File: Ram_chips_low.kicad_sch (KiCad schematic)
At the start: 10 parts, among them U25 MM5280, U26 MM5280, U27 MM5280, U28 MM5280, U40 MM5280, U41 MM5280, U42 MM5280, U43 MM5280, U6 74LS04, U7 74LS173

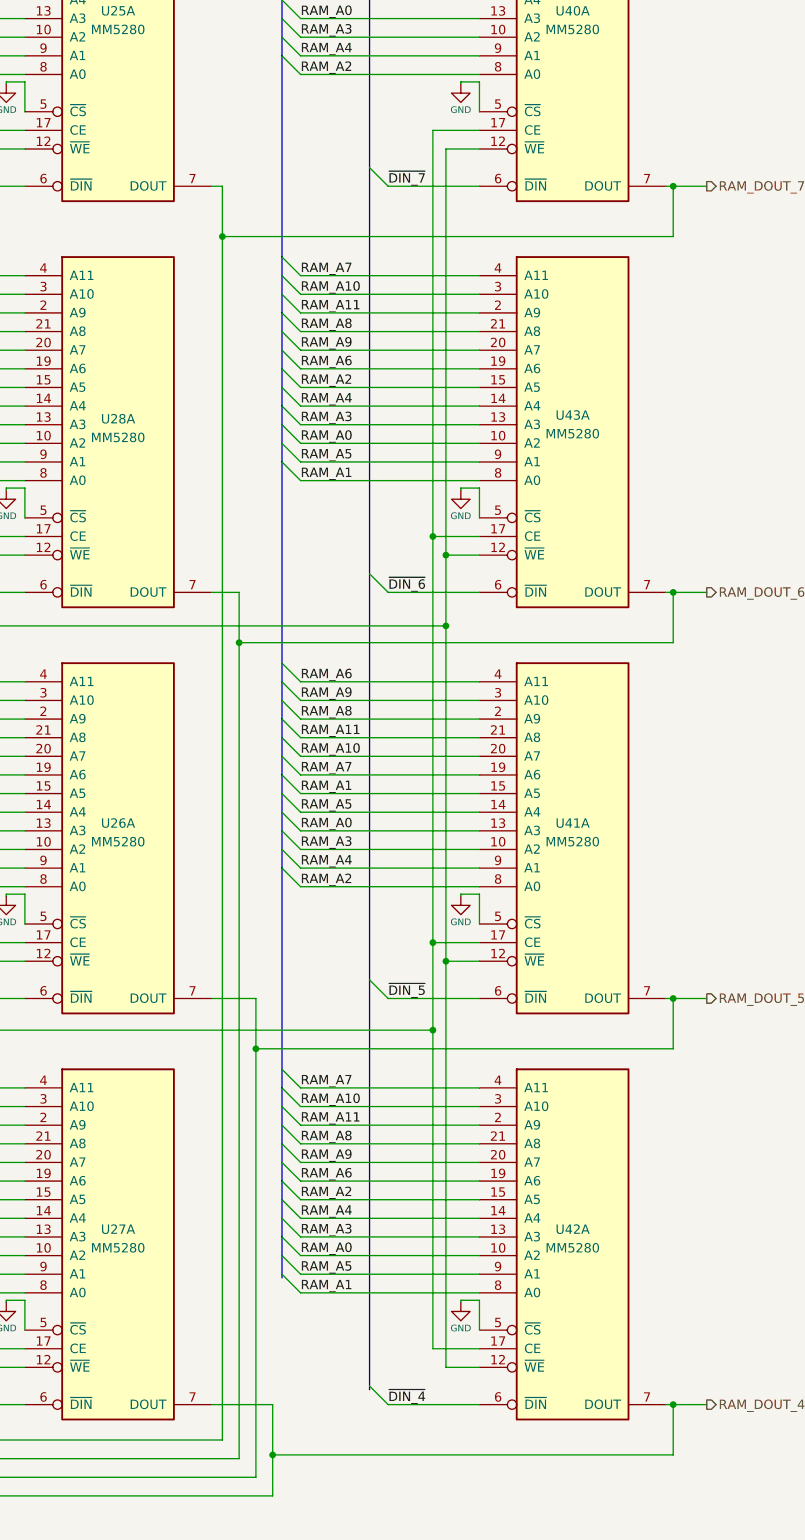
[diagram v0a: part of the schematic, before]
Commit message: Routing completed
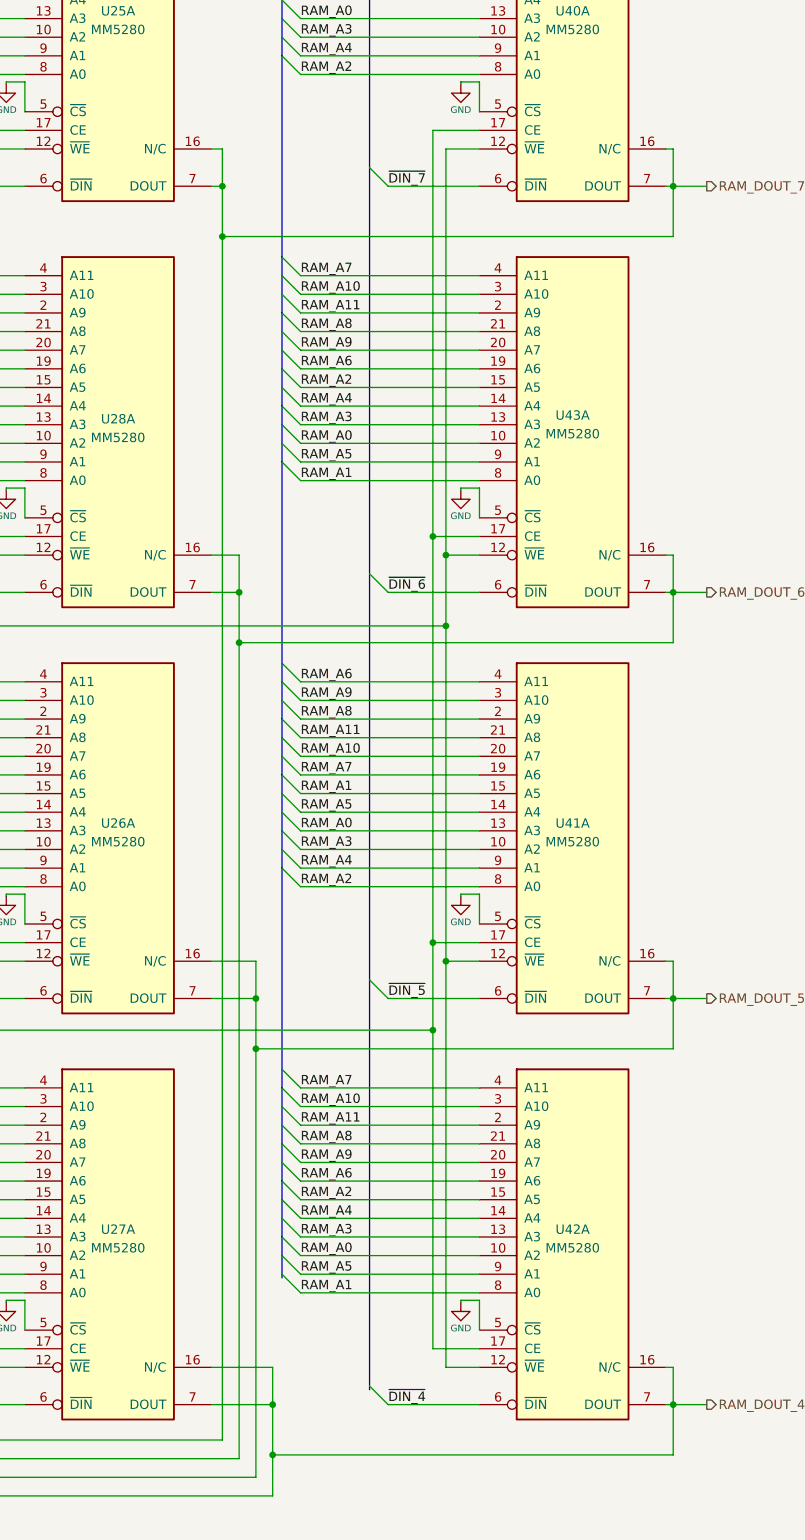
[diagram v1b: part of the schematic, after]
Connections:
- net RAM_DOUT_4: now also U27.16 (N/C), U42.16 (N/C)
- net RAM_DOUT_5: now also U26.16 (N/C), U41.16 (N/C)
- net RAM_DOUT_6: now also U28.16 (N/C), U43.16 (N/C)
- net RAM_DOUT_7: now also U25.16 (N/C), U40.16 (N/C)
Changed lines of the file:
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@@
   (junction (at 146.05 127.508) (diameter 0) (color 0 0 0 0)
   )
+  (junction (at 120.142 178.308) (diameter 0) (color 0 0 0 0)
+  )
+  (junction (at 117.856 122.936) (diameter 0) (color 0 0 0 0)
+  )
   (junction (at 120.142 185.166) (diameter 0) (color 0 0 0 0)
   )
+  (junction (at 122.428 233.68) (diameter 0) (color 0 0 0 0)
+  )
   (junction (at 81.534 115.316) (diameter 0) (color 0 0 0 0)
   )
@@
   (junction (at 33.274 195.072) (diameter 0) (color 0 0 0 0)
   )
+  (junction (at 115.57 67.564) (diameter 0) (color 0 0 0 0)
+  )
   (junction (at 83.312 117.856) (diameter 0) (color 0 0 0 0)
   )
@@
     (stroke (width 0) (type default))
   )
+  (wire (pts (xy 120.142 173.228) (xy 120.142 178.308))
+    (stroke (width 0) (type default))
+  )
   (wire (pts (xy 83.312 173.228) (xy 88.646 173.228))
     (stroke (width 0) (type default))
@@
     (stroke (width 0) (type default))
   )
+  (wire (pts (xy 177.038 173.228) (xy 177.038 178.308))
+    (stroke (width 0) (type default))
+  )
   (wire (pts (xy 126.238 82.296) (xy 150.622 82.296))
     (stroke (width 0) (type default))
   )
+  (wire (pts (xy 177.038 62.484) (xy 177.038 67.564))
+    (stroke (width 0) (type default))
+  )
   (bus (pts (xy 60.452 208.28) (xy 60.452 210.82))
     (stroke (width 0) (type default))
@@
     (stroke (width 0) (type default))
   )
+  (wire (pts (xy 176.022 173.228) (xy 177.038 173.228))
+    (stroke (width 0) (type default))
+  )
   (bus (pts (xy 60.452 77.216) (xy 60.452 79.756))
     (stroke (width 0) (type default))
@@
     (stroke (width 0) (type default))
   )
+  (wire (pts (xy 176.022 228.6) (xy 177.038 228.6))
+    (stroke (width 0) (type default))
+  )
   (bus (pts (xy 60.452 102.616) (xy 60.452 105.156))
     (stroke (width 0) (type default))
@@
     (stroke (width 0) (type default))
   )
+  (wire (pts (xy 114.046 228.6) (xy 122.428 228.6))
+    (stroke (width 0) (type default))
+  )
   (wire (pts (xy 62.992 195.58) (xy 88.646 195.58))
     (stroke (width 0) (type default))
@@
     (stroke (width 0) (type default))
   )
+  (wire (pts (xy 115.57 62.484) (xy 115.57 67.564))
+    (stroke (width 0) (type default))
+  )
   (bus (pts (xy 60.452 29.464) (xy 60.452 30.988))
     (stroke (width 0) (type default))
@@
     (stroke (width 0) (type default))
   )
+  (wire (pts (xy 176.022 62.484) (xy 177.038 62.484))
+    (stroke (width 0) (type default))
+  )
   (bus (pts (xy 123.698 203.2) (xy 123.698 205.74))
     (stroke (width 0) (type default))
@@
     (stroke (width 0) (type default))
   )
+  (wire (pts (xy 114.046 117.856) (xy 117.856 117.856))
+    (stroke (width 0) (type default))
+  )
   (wire (pts (xy 62.992 147.828) (xy 88.646 147.828))
     (stroke (width 0) (type default))
@@
     (stroke (width 0) (type default))
   )
+  (wire (pts (xy 177.038 228.6) (xy 177.038 233.68))
+    (stroke (width 0) (type default))
+  )
   (wire (pts (xy 88.646 115.316) (xy 81.534 115.316))
     (stroke (width 0) (type default))
@@
     (stroke (width 0) (type default))
   )
+  (wire (pts (xy 122.428 228.6) (xy 122.428 233.68))
+    (stroke (width 0) (type default))
+  )
   (wire (pts (xy 33.782 279.4) (xy 83.312 279.4))
     (stroke (width 0) (type default))
@@
     (stroke (width 0) (type default))
   )
+  (wire (pts (xy 176.022 117.856) (xy 177.038 117.856))
+    (stroke (width 0) (type default))
+  )
   (bus (pts (xy 60.452 36.068) (xy 60.452 37.084))
     (stroke (width 0) (type default))
@@
     (stroke (width 0) (type default))
   )
+  (wire (pts (xy 177.038 117.856) (xy 177.038 122.936))
+    (stroke (width 0) (type default))
+  )
   (wire (pts (xy 138.176 67.564) (xy 150.622 67.564))
     (stroke (width 0) (type default))
@@
     (stroke (width 0) (type default))
   )
+  (wire (pts (xy 117.856 117.856) (xy 117.856 122.936))
+    (stroke (width 0) (type default))
+  )
   (wire (pts (xy 126.238 137.668) (xy 150.622 137.668))
     (stroke (width 0) (type default))
@@
     (stroke (width 0) (type default))
   )
+  (wire (pts (xy 114.046 173.228) (xy 120.142 173.228))
+    (stroke (width 0) (type default))
+  )
   (bus (pts (xy 123.698 29.464) (xy 123.698 26.924))
     (stroke (width 0) (type default))
@@
     (stroke (width 0) (type default))
   )
+  (wire (pts (xy 114.046 62.484) (xy 115.57 62.484))
+    (stroke (width 0) (type default))
+  )
